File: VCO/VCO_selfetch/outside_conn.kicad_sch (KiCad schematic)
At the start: 24 parts

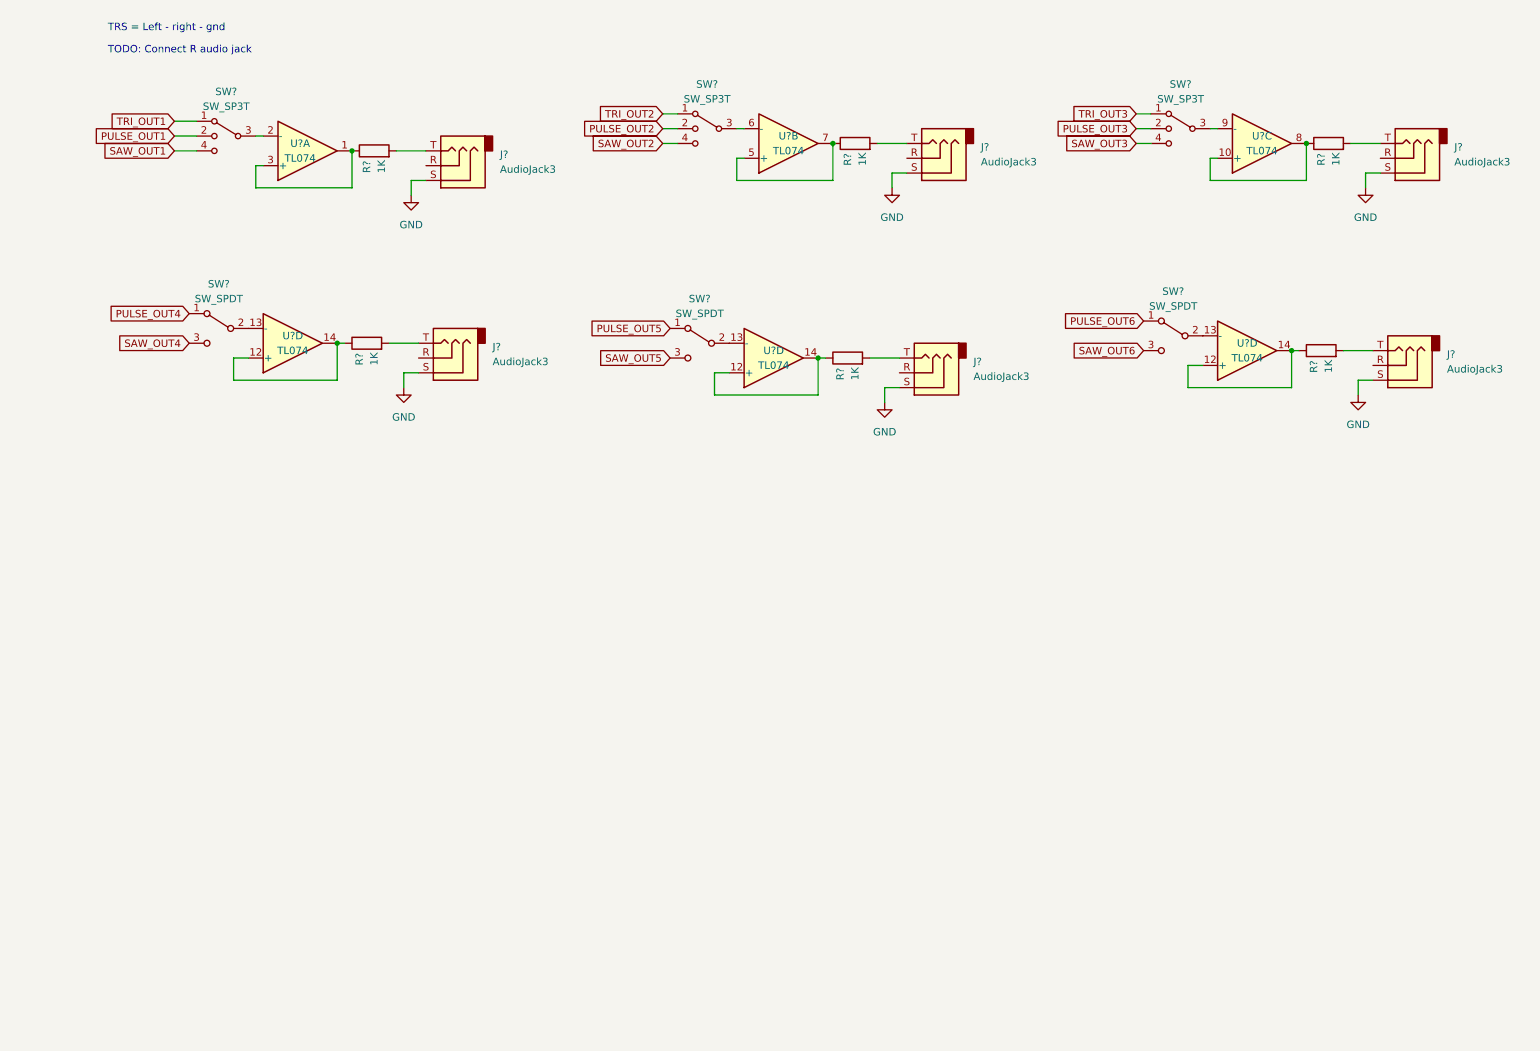
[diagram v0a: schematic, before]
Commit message: continue
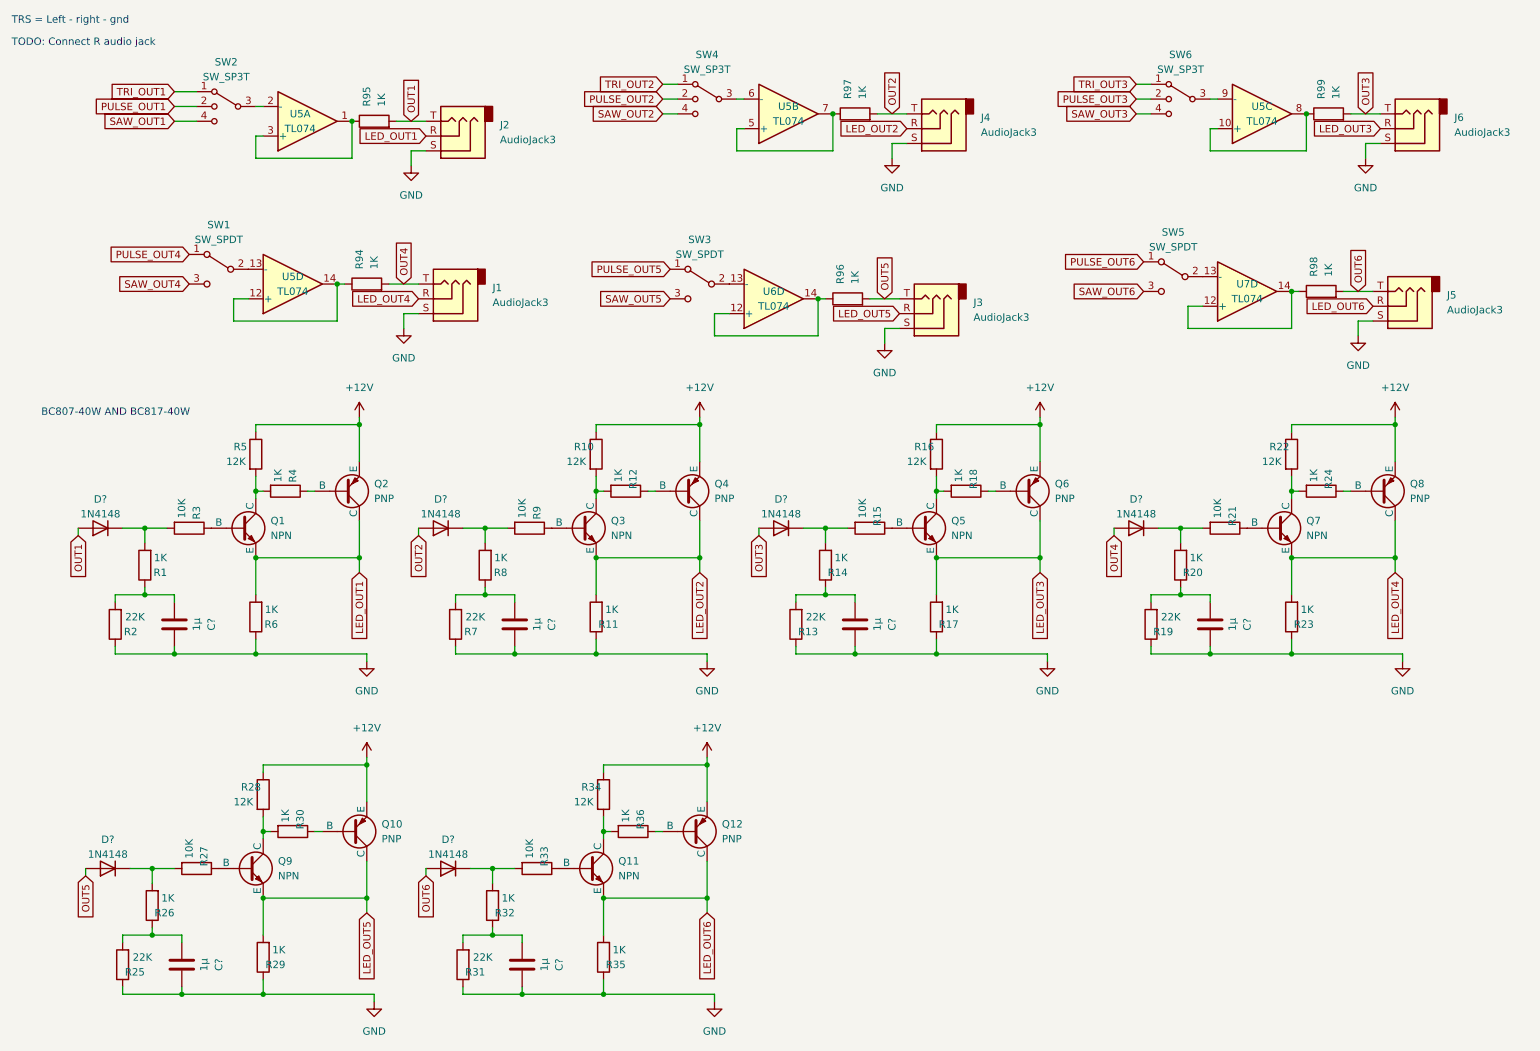
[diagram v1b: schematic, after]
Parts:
- added C? (x6): 1µ, symbol Device:C
- added D? (x6): 1N4148, Diode_THT:D_DO-35_SOD27_P7.62mm_Horizontal, symbol Diode:1N4148
- added Q1, Q11, Q3, Q5, Q7, Q9: NPN, symbol Simulation_SPICE:NPN
- added Q10, Q12, Q2, Q4, Q6, Q8: PNP, symbol Simulation_SPICE:PNP
- added R1, R11, R12, R14, R17, R18, R20, R23, R24, R26, R29, R30, R32, R35, R36, R4, R6, R8: 1K, symbol Device:R
- added R10, R16, R22, R28, R34, R5: 12K, symbol Device:R
- added R13, R19, R2, R25, R31, R7: 22K, symbol Device:R
- added R15, R21, R27, R3, R33, R9: 10K, symbol Device:R
- gave numbers to parts that had none: 21
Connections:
- net GND: now also C?.1, C?.1, C?.1, C?.1, C?.1, C?.1, R11.1, R13.1, R17.1, R19.1, R2.1, R23.1, R25.1, R29.1, R31.1, R35.1, R6.1, R7.1
- net OUT3: now reaches J6.T, R99.2
- net OUT3: now also D?.2 (A)
- net LED_OUT3: now reaches J6.R
- net LED_OUT3: now also Q5.3 (E), Q6.1 (C), R17.2
- net LED_OUT1: now reaches J2.R
- net LED_OUT1: now also Q1.3 (E), Q2.1 (C), R6.2
- net OUT1: now reaches J2.T, R95.2
- net OUT1: now also D?.2 (A)
- net OUT4: now reaches J1.T, R94.2
- net OUT4: now also D?.2 (A)
- net OUT2: now reaches J4.T, R97.2
- net OUT2: now also D?.2 (A)
- net OUT6: now reaches J5.T, R98.2
- net OUT6: now also D?.2 (A)
- net LED_OUT5: now reaches J3.R
- net LED_OUT5: now also Q10.1 (C), Q9.3 (E), R29.2
- net OUT5: now reaches J3.T, R96.2
- net OUT5: now also D?.2 (A)
- net LED_OUT4: now reaches J1.R
- net LED_OUT4: now also Q7.3 (E), Q8.1 (C), R23.2
- net LED_OUT6: now reaches J5.R
- net LED_OUT6: now also Q11.3 (E), Q12.1 (C), R35.2
- net LED_OUT2: now reaches J4.R
- net LED_OUT2: now also Q3.3 (E), Q4.1 (C), R11.2
- new net: D?.1 (K), R8.2, R9.2
- new net: Q7.1 (C), R22.2, R24.2
- new net: Q12.2 (B), R36.1
- new net: D?.1 (K), R20.2, R21.2
- new net: C?.2, R31.2, R32.1
- new net: D?.1 (K), R32.2, R33.2
- new net: C?.2, R7.2, R8.1
- new net: C?.2, R25.2, R26.1
- new net: D?.1 (K), R26.2, R27.2
- new net: Q1.1 (C), R4.2, R5.2
- new net: Q6.2 (B), R18.1
- new net: C?.2, R19.2, R20.1
- new net: Q4.2 (B), R12.1
- new net: Q11.2 (B), R33.1
- new net: Q9.1 (C), R28.2, R30.2
- new net: Q9.2 (B), R27.1
- new net: C?.2, R13.2, R14.1
- new net: D?.1 (K), R14.2, R15.2
- new net: Q8.2 (B), R24.1
- new net: Q5.2 (B), R15.1
- new net: Q5.1 (C), R16.2, R18.2
- new net: Q11.1 (C), R34.2, R36.2
- new net: Q10.2 (B), R30.1
- new net: Q1.2 (B), R3.1
- new net: D?.1 (K), R1.2, R3.2
- new net: C?.2, R1.1, R2.2
- new net: Q3.1 (C), R10.2, R12.2
- new net: Q3.2 (B), R9.1
- new net: Q7.2 (B), R21.1
- new net: Q2.2 (B), R4.1
- new net +12V: Q10.3 (E), Q12.3 (E), Q2.3 (E), Q4.3 (E), Q6.3 (E), Q8.3 (E), R10.1, R16.1, R22.1, R28.1, R34.1, R5.1
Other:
- note added: "BC807-40W AND BC817-40W"
- moved on the sheet: J1, J2, J3, J4, J5, J6, R94, R95, R96, R97, R98, R99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
